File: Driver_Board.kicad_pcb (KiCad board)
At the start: 4 copper layers, 32 parts, among them J1 Conn_02x07_Odd_Even, J2 IGBT, J3 IGBT_Diode, J4 Conn_01x01, U1 TEC2-1213WI

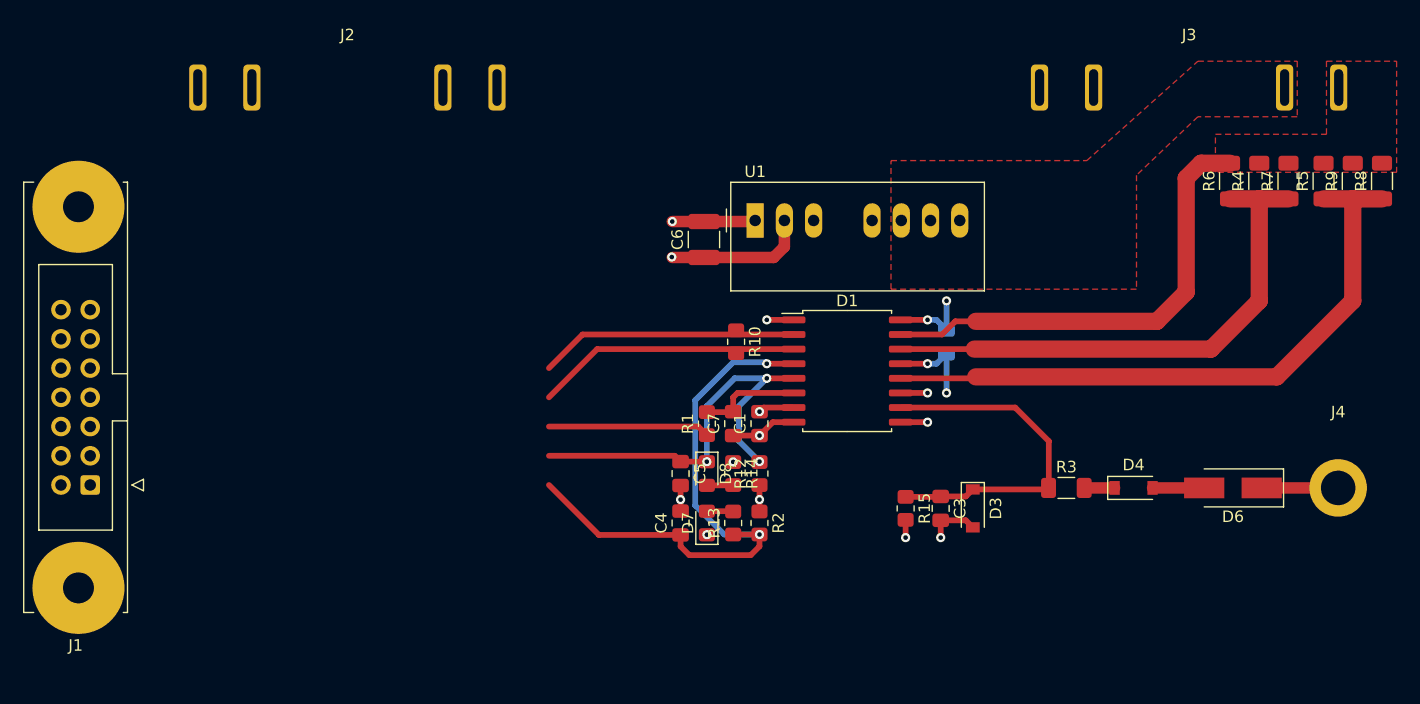
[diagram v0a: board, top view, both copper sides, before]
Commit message: Первая версия в производство
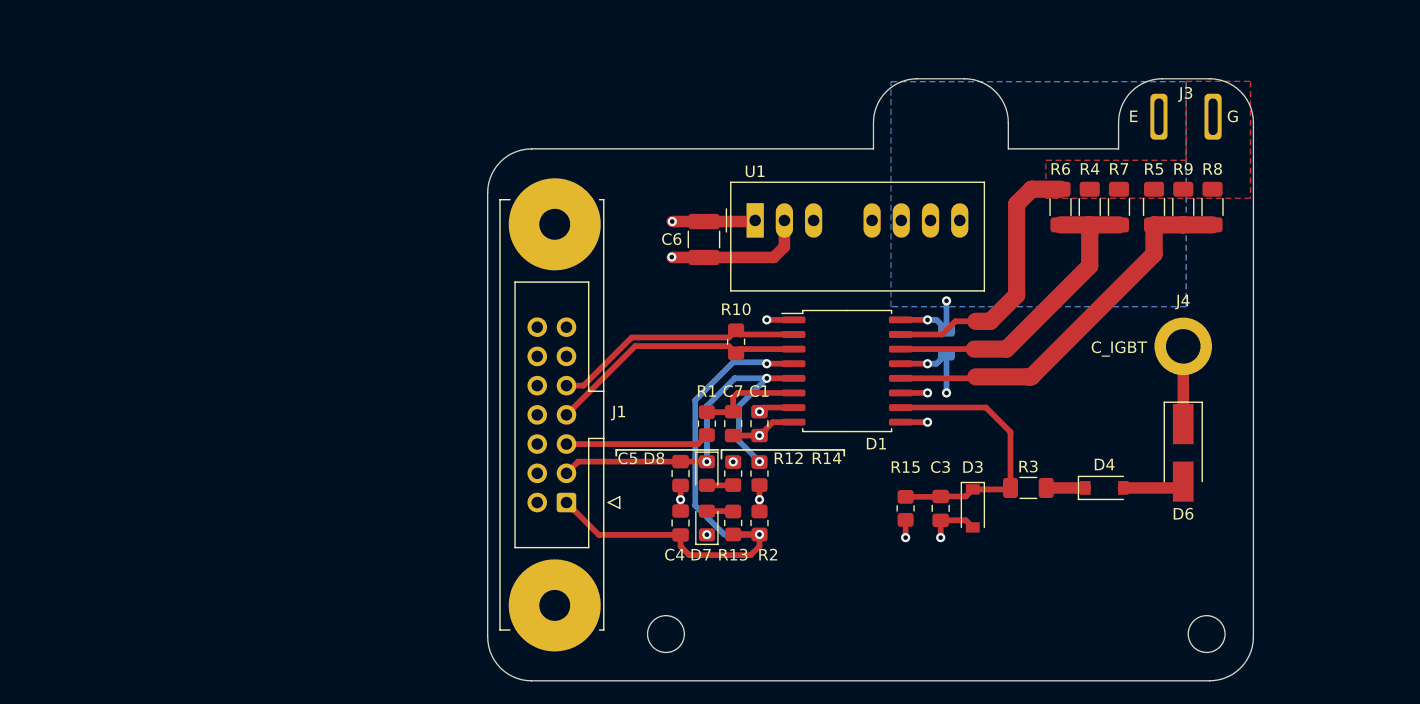
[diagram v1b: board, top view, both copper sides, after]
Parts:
- removed J2: IGBT, IGBT_Modul:IGBT_Gate
- added H1: MountingHole, MountingHole:MountingHole_3.2mm_M3, F.Cu at (120.7, 97.0)
- added H3: MountingHole, MountingHole:MountingHole_3.2mm_M3, F.Cu at (73.7, 97.0)
- moved J1 41.4 mm to (65.0, 85.6)
- moved J4 18.2 mm to (118.6, 65.9)
- moved R4 14.9 mm to (110.5, 59.9)
- moved R5 14.9 mm to (116.1, 59.9)
- moved R6 14.9 mm to (108.0, 59.9)
- moved R7 14.9 mm to (113.0, 59.9)
- moved R9 14.9 mm to (118.6, 59.9)
- moved R8 14.9 mm to (121.2, 59.9)
- moved J3 11.2 mm to (108.2, 52.1)
- moved D6 5.29 mm to (118.6, 81.3), turned to -90 degrees
- moved R3 3.30 mm to (105.2, 84.3)
- moved D4 2.54 mm to (111.8, 84.3)
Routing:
- net Net-(D1-Pad12): track 56.0 -> 34.1 mm
- net Net-(D1-Pad14): track 46.8 -> 28.1 mm
- net G_IGBT: track 40.6 -> 23.7 mm
- net Desat: track 30.9 -> 24.7 mm
- net RDY: track 51.0 -> 48.6 mm
- net RST: track 14.0 -> 12.5 mm
- net FLT: track 36.3 -> 35.0 mm
- net Net-(D4-Pad2): track 4.49 -> 5.43 mm
- net Net-(D4-Pad1): track 2.64 -> 3.40 mm
- net IN+: track 22.5 -> 21.9 mm
- added copper zone on B.Cu, net E_IGBT
- removed copper zone on F.Cu, net E_IGBT
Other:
- board outline added: 66.5 x 52.3 mm
- board text added: "C_IGBT"
- board text added: "E"
- board text added: "G"
